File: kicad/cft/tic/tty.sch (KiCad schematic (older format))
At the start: 40 parts, among them J601 DE9-Female-with-Shield, J602 DE9-Female-with-Shield, J603 USB_OTG, U601 MAX232, U602 STC16C554, U603 MAX232, U604 MAX232, U605 MAX232, U606 FT231XS, X601 7.3728 MHz

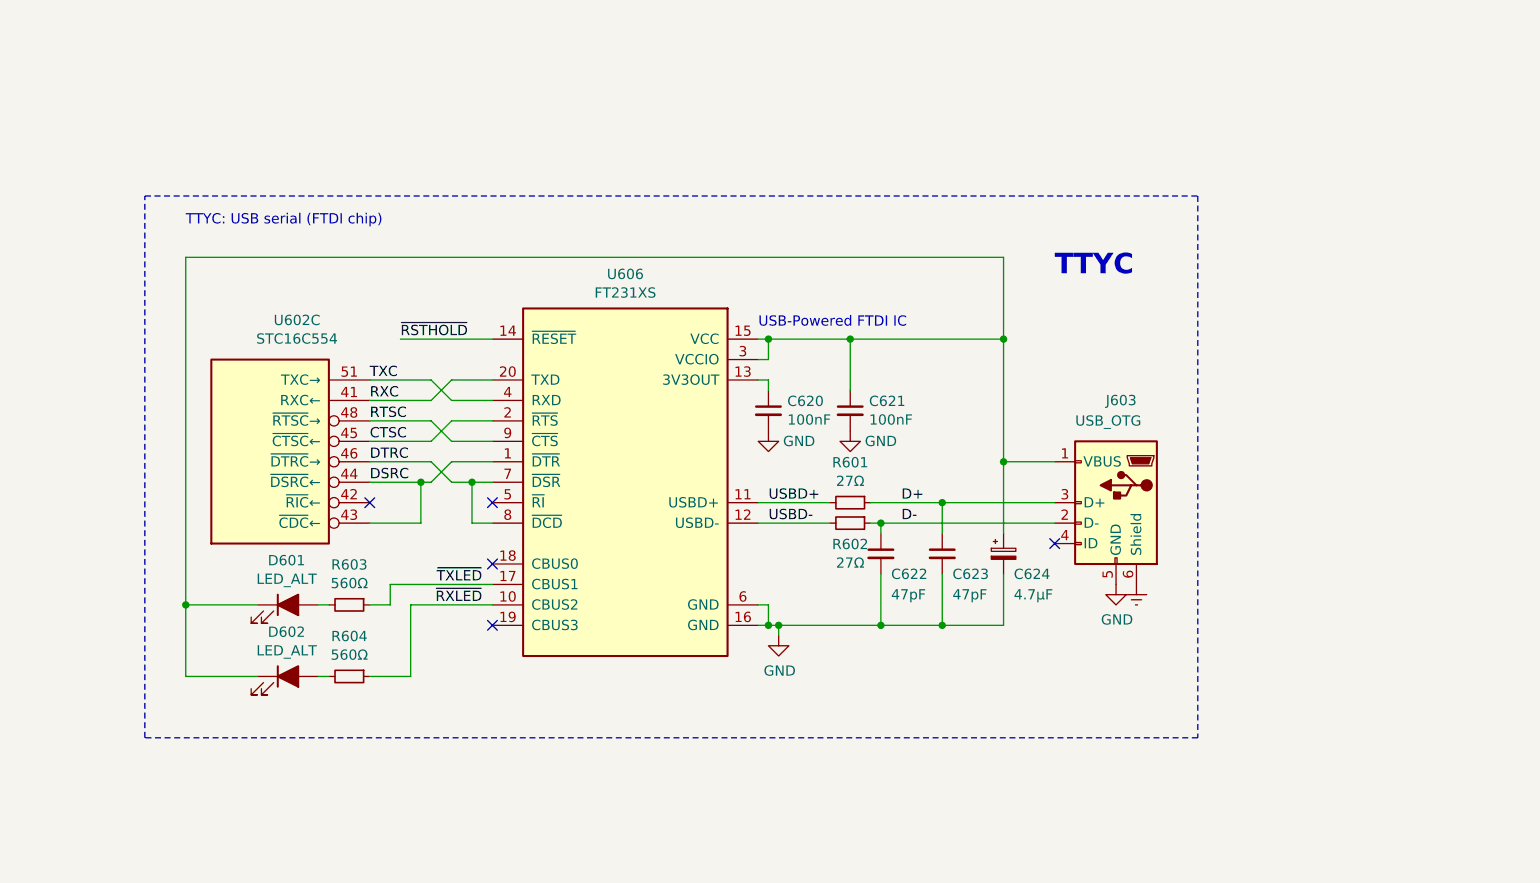
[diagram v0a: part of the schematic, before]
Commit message: Work on TIC board
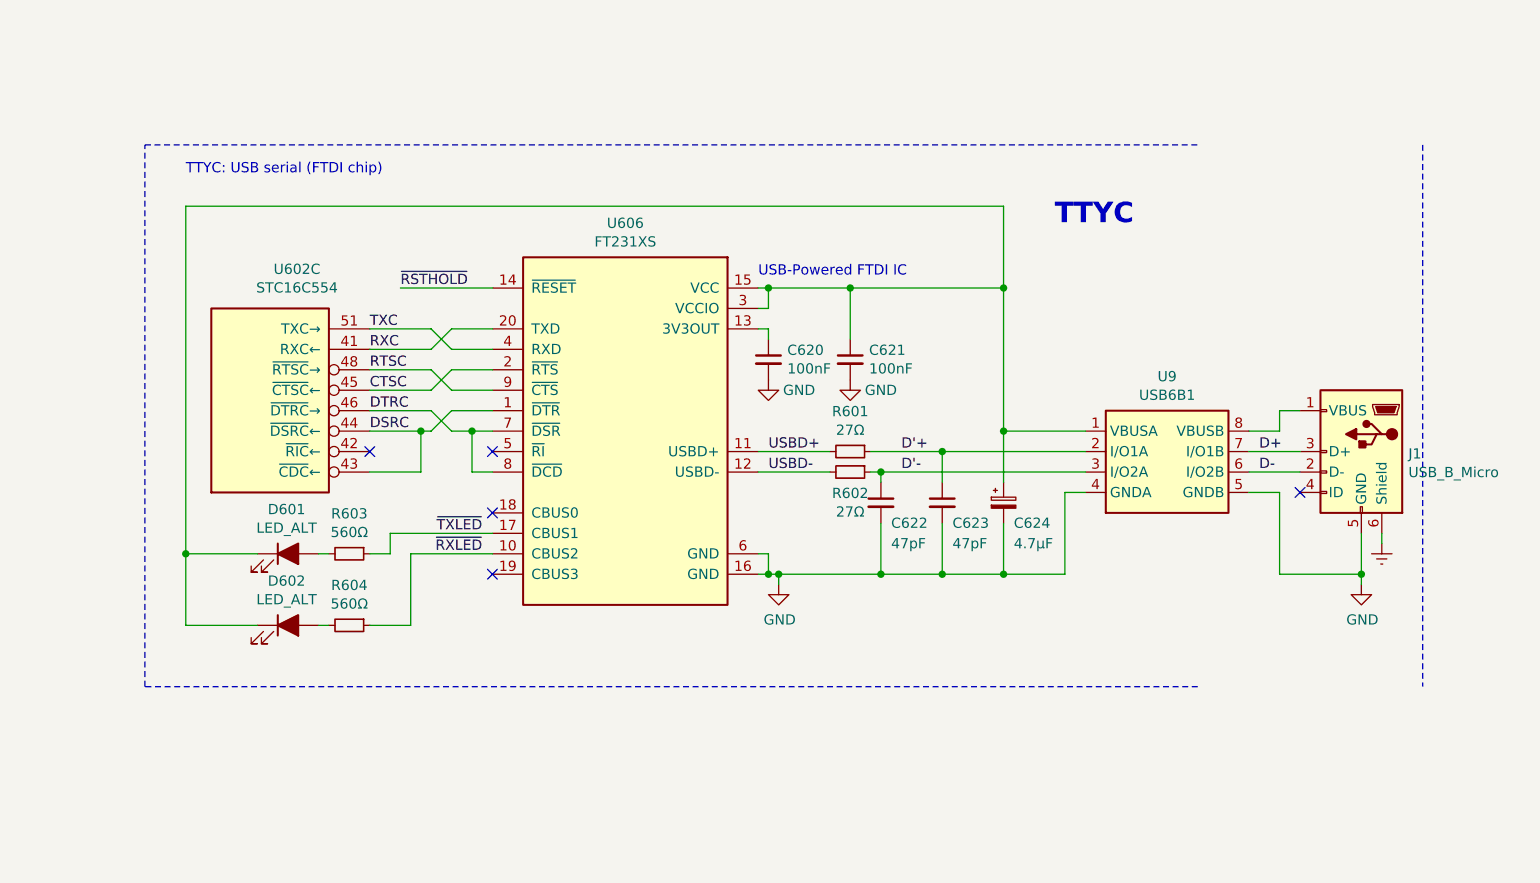
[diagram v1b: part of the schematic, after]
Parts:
- removed J603: USB_OTG, Connector_USB:USB_B_Lumberg_2411_02_Horizontal, symbol Connector:USB_OTG
- added J1: USB_B_Micro, Connector_USB:USB_Micro-B_Molex_47346-0001, symbol Connector:USB_B_Micro
- added U9: USB6B1, alexios:SOIC-8, symbol alexios:USB6B1
- U601, U603, U605: footprint Package_DIP:DIP-16_W7.62mm_Socket -> alexios:DIP-16_W7.62mm_Socket
- U602: footprint Package_LCC:PLCC-68 -> alexios:PLCC68
- U604: footprint Package_LCC:PLCC-68_THT-Socket -> alexios:DIP-16_W7.62mm_Socket
- U606: footprint Housings_SSOP:SSOP-20_4.4x6.5mm_Pitch0.65mm -> Package_SO:SSOP-20_3.9x8.7mm_P0.635mm
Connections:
- net D+: now also J1.3 (D+), U9.7 (I/O1B); no longer C623.1, R601.1
- net D-: now also J1.2 (D-), U9.6 (I/O2B); no longer C622.1, R602.1
- net Earth: now also J1.6 (Shield)
- net GND: now also J1.5 (GND), U9.4 (GNDA), U9.5 (GNDB)
- net at C621.1, C624.1, D601.1 (K)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: now also U9.1 (VBUSA)
- new net: J1.1 (VBUS), U9.8 (VBUSB)
- new net D'+: C623.1, R601.1, U9.2 (I/O1A)
- new net D'-: C622.1, R602.1, U9.3 (I/O2A)
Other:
- moved on the sheet: C620, C621, C622, C623, C624, D601, D602, R601, R602, R603, R604, U602C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
